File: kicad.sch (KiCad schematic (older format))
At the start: 18 parts, among them J1 Screw_Terminal_01x03, J2 Conn_01x05, J3 ICSP, SW1 SW_Push, SW2 SW_Push, U1 ADS1115IDGS, U2 ADS1115IDGS, U3 ESP-12E

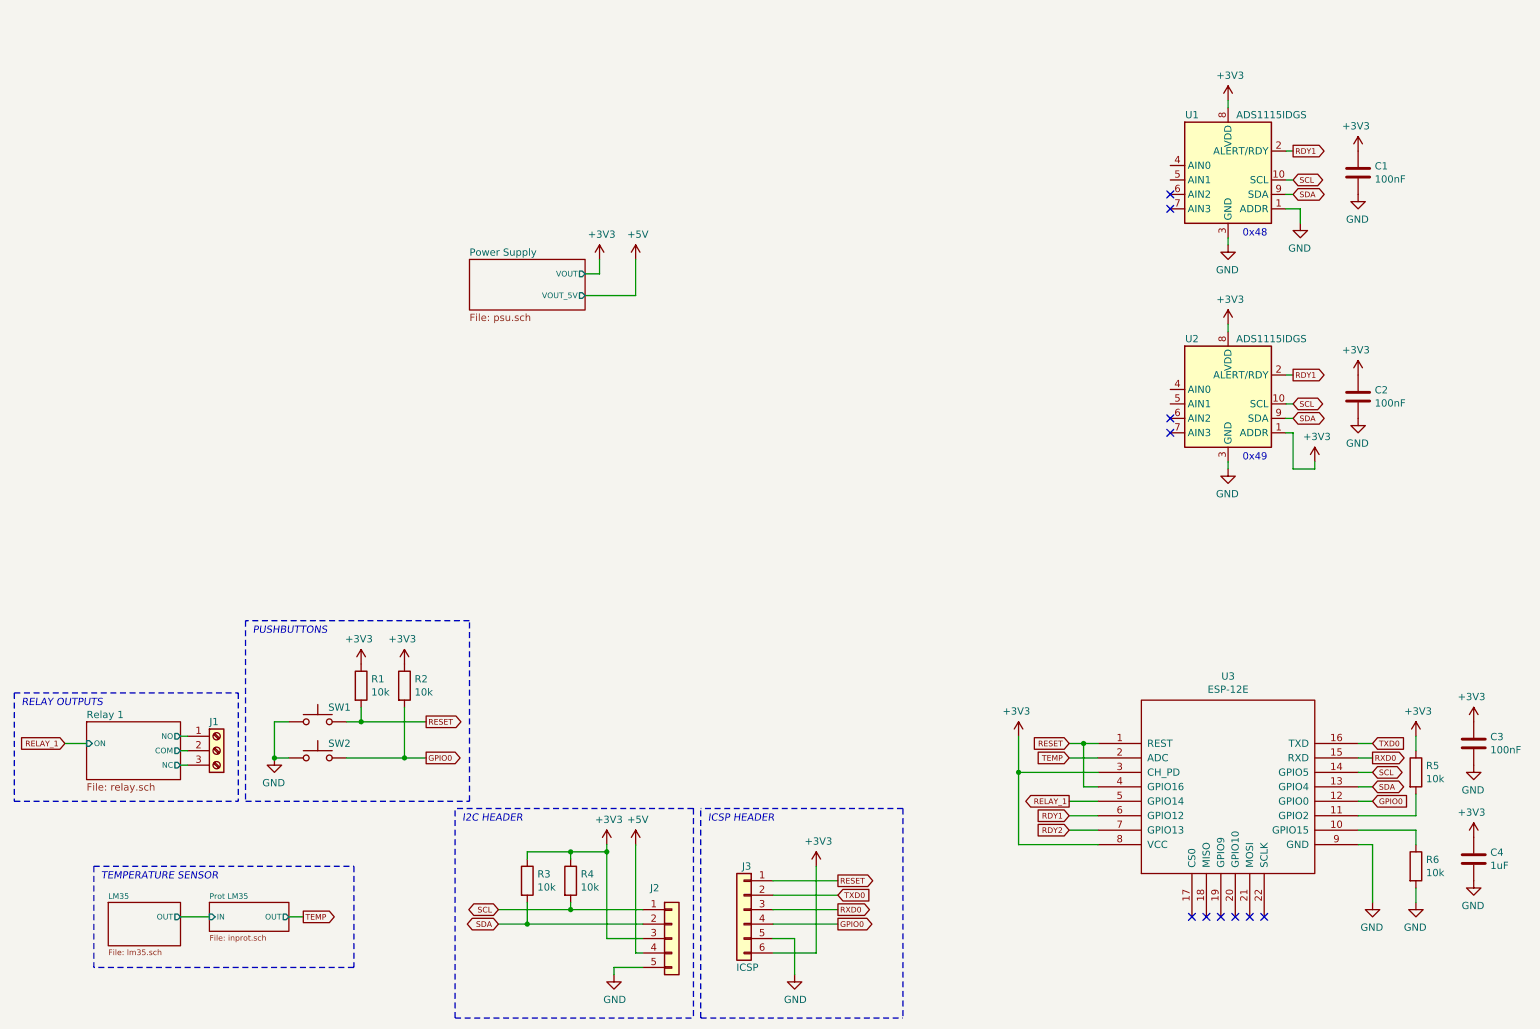
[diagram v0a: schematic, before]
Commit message: quiero dormir culiaaaa
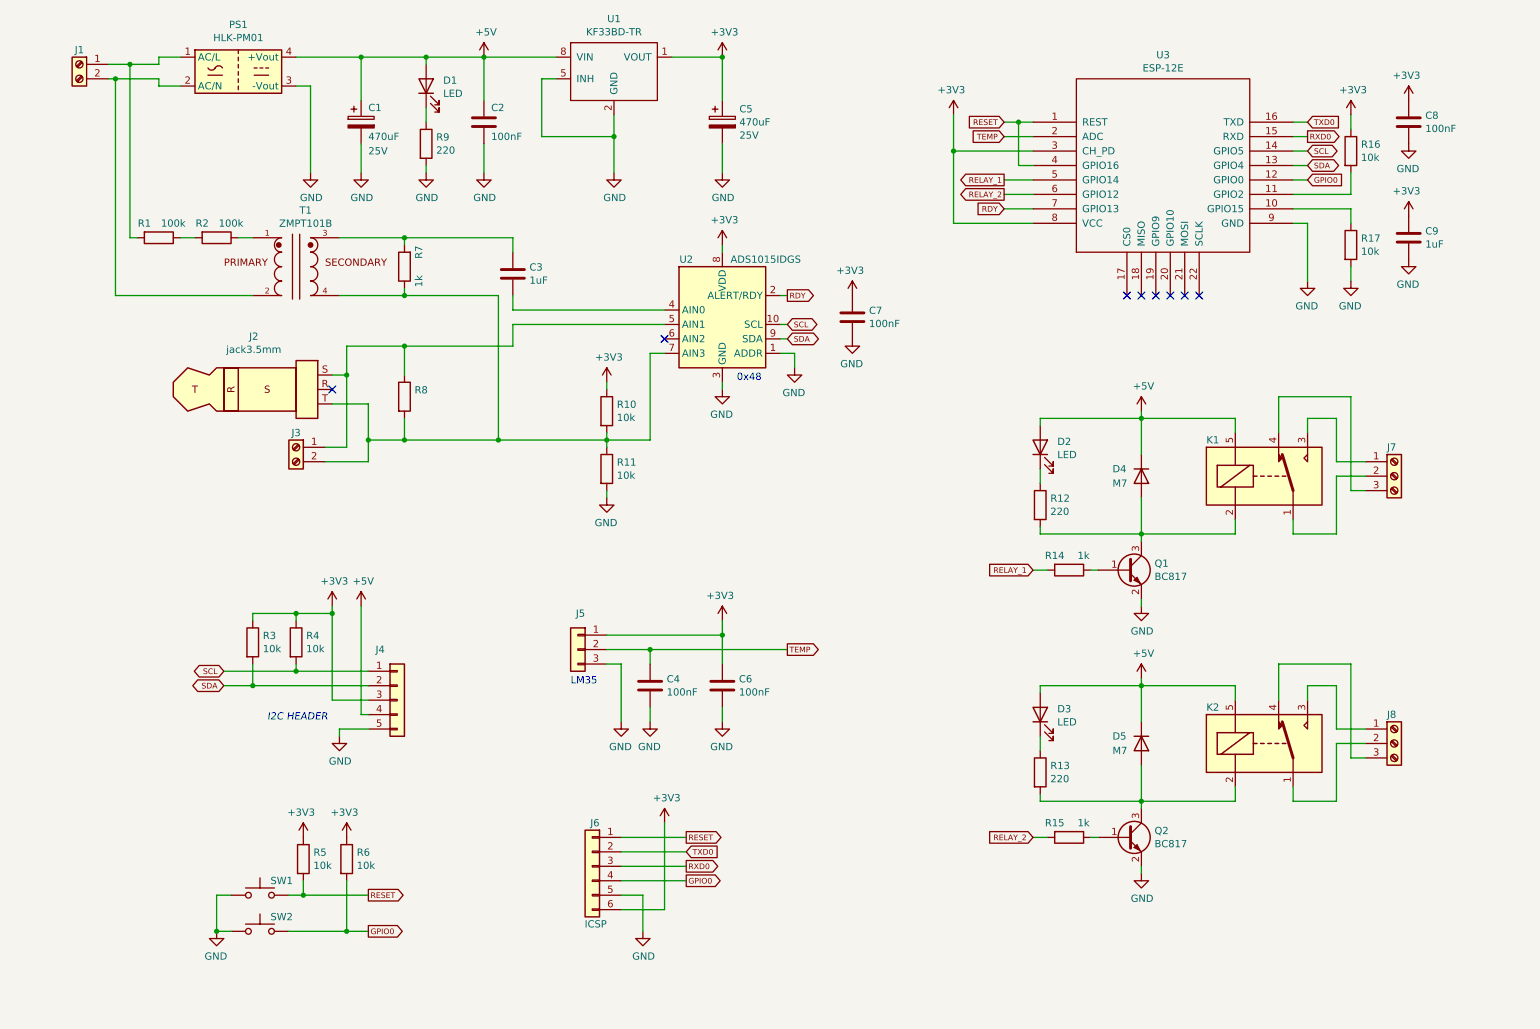
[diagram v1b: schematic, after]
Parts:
- removed U1, U2: ADS1115IDGS, Package_SO:TSSOP-10_3x3mm_P0.5mm, symbol Analog_ADC:ADS1115IDGS
- added C1, C5: 470uF, libs:CAP_10x10_SMD_THT, symbol Device:CP
- added C3: 1uF, Capacitor_SMD:C_1206_3216Metric_Pad1.33x1.80mm_HandSolder, symbol Device:C
- added C4, C6: 100nF, Capacitor_SMD:C_1206_3216Metric_Pad1.33x1.80mm_HandSolder, symbol Device:C
- added D1, D2, D3: LED, LED_SMD:LED_1206_3216Metric, symbol Device:LED
- added D4, D5: M7, Diode_SMD:D_SMA_Handsoldering, symbol Diode:1N4007
- added J1, J3: Screw_Terminal_01x02, libs:TerminalBlock_bornier-2_P5.08mm, symbol Connector:Screw_Terminal_01x02
- added J2: jack3.5mm, Connector_Audio:Jack_3.5mm_Ledino_KB3SPRS_Horizontal, symbol Connector:AudioPlug3
- added J5: Conn_01x03, Connector_Molex:Molex_KK-254_AE-6410-03A_1x03_P2.54mm_Vertical, symbol Connector_Generic:Conn_01x03
- added J7: Screw_Terminal_01x03, libs:TerminalBlock_bornier-3_P5.08mm, symbol Connector:Screw_Terminal_01x03
- added K1, K2: RELAY 0510, Relay_THT:Relay_SPDT_SANYOU_SRD_Series_Form_C, symbol Relay:SANYOU_SRD_Form_C
- added PS1: HLK-PM01, Converter_ACDC:Converter_ACDC_HiLink_HLK-PMxx, symbol Converter_ACDC:HLK-PM01
- added Q1, Q2: BC817, Package_TO_SOT_SMD:SOT-23, symbol Transistor_BJT:BC817
- added R1, R2: 100k, Resistor_SMD:R_1206_3216Metric, symbol Device:R
- added R10, R11: 10k, Resistor_SMD:R_1206_3216Metric, symbol Device:R
- added R12, R13, R9: 220, Resistor_SMD:R_1206_3216Metric, symbol Device:R
- added R14, R15, R7: 1k, Resistor_SMD:R_1206_3216Metric, symbol Device:R
- added R8: ?, Resistor_SMD:R_1206_3216Metric, symbol Device:R
- added T1: ZMPT101B, ZMPT101B:ZMPT101B, symbol ZMPT101B:ZMPT101B
- added U1: KF33BD-TR, Package_SO:SO-8_3.9x4.9mm_P1.27mm, symbol kf33:KF33BD-TR
- added U2: ADS1015IDGS, Package_SO:TSSOP-10_3x3mm_P0.5mm, symbol Analog_ADC:ADS1015IDGS
- renumbered C1 to C7, C3 to C8, C4 to C9, J2 to J4, J3 to J6, J1 to J8, R5 to R16, R6 to R17, R1 to R5, R2 to R6
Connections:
- net +3V3: now also C5.1, C6.1, J5.1 (Pin_1), R10.1, U1.1 (VOUT), U2.8 (VDD); no longer C2.1
- net +5V: now also C2.1, C1.1, D1.2 (A), D2.2 (A), D3.2 (A), D4.1 (K), D5.1 (K), K1.5, K2.5, PS1.4 (+Vout), U1.8 (VIN)
- net GND: now also C1.2, C4.2, C5.2, C6.2, J5.3 (Pin_3), PS1.3 (-Vout), Q1.2 (E), Q2.2 (E), R11.2, R9.2, U1.2 (GND), U1.3 (GND), U1.5 (INH), U1.6 (GND), U1.7 (GND), U2.1 (ADDR), U2.3 (GND)
- net RELAY_1: now also R14.2
- net SCL: now also U2.10 (SCL)
- net SDA: now also U2.9 (SDA)
- net TEMP: now also C4.1, J5.2 (Pin_2)
- net RDY1 renamed RELAY_2
- net RELAY_2: now also R15.2
- net RDY2 renamed RDY
- net RDY: now also U2.2 (ALERT/RDY)
- net Relay 1/COM: no longer names the net of J8.2 (Pin_2)
- net Relay 1/COM: now also K2.1
- net Relay 1/NC: no longer names the net of J8.3 (Pin_3)
- net Relay 1/NC: now also K2.4
- net Relay 1/NO: no longer names the net of J8.1 (Pin_1)
- net Relay 1/NO: now also K2.3
- new net: Q2.1 (B), R15.1
- new net: D5.2 (A), K2.2, Q2.3 (C), R13.2
- new net: D3.1 (K), R13.1
- new net: D1.1 (K), R9.1
- new net: J1.1 (Pin_1), PS1.1 (AC/L), R1.2
- new net: J1.2 (Pin_2), PS1.2 (AC/N), T1.2
- new net: C3.2, U2.4 (AIN0)
- new net: J2.S, J3.1 (Pin_1), R8.1, U2.5 (AIN1)
- new net: J2.T, J3.2 (Pin_2), R10.2, R11.1, R7.1, R8.2, T1.4, U2.7 (AIN3)
- new net: J7.1 (Pin_1), K1.3
- new net: J7.2 (Pin_2), K1.1
- new net: J7.3 (Pin_3), K1.4
- new net: Q1.1 (B), R14.1
- new net: D4.2 (A), K1.2, Q1.3 (C), R12.2
- new net: D2.1 (K), R12.1
- new net: R2.1, T1.1
- new net: C3.1, R7.2, T1.3
- new net: R1.1, R2.2
- no-connect marks 10 -> 8
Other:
- note added: "LM35"
- note removed: "0x49"
- note removed: "ICSP HEADER"
- note removed: "PUSHBUTTONS"
- note removed: "RELAY OUTPUTS"
- note removed: "TEMPERATURE SENSOR"
- moved on the sheet: C7, C8, C9, J4, J6, J8, R16, R17, R3, R4, R5, R6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
